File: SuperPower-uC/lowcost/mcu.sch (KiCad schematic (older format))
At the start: 5 parts, among them J5 main pin header, J6 main pin header, U13 ESP32-WROOM32

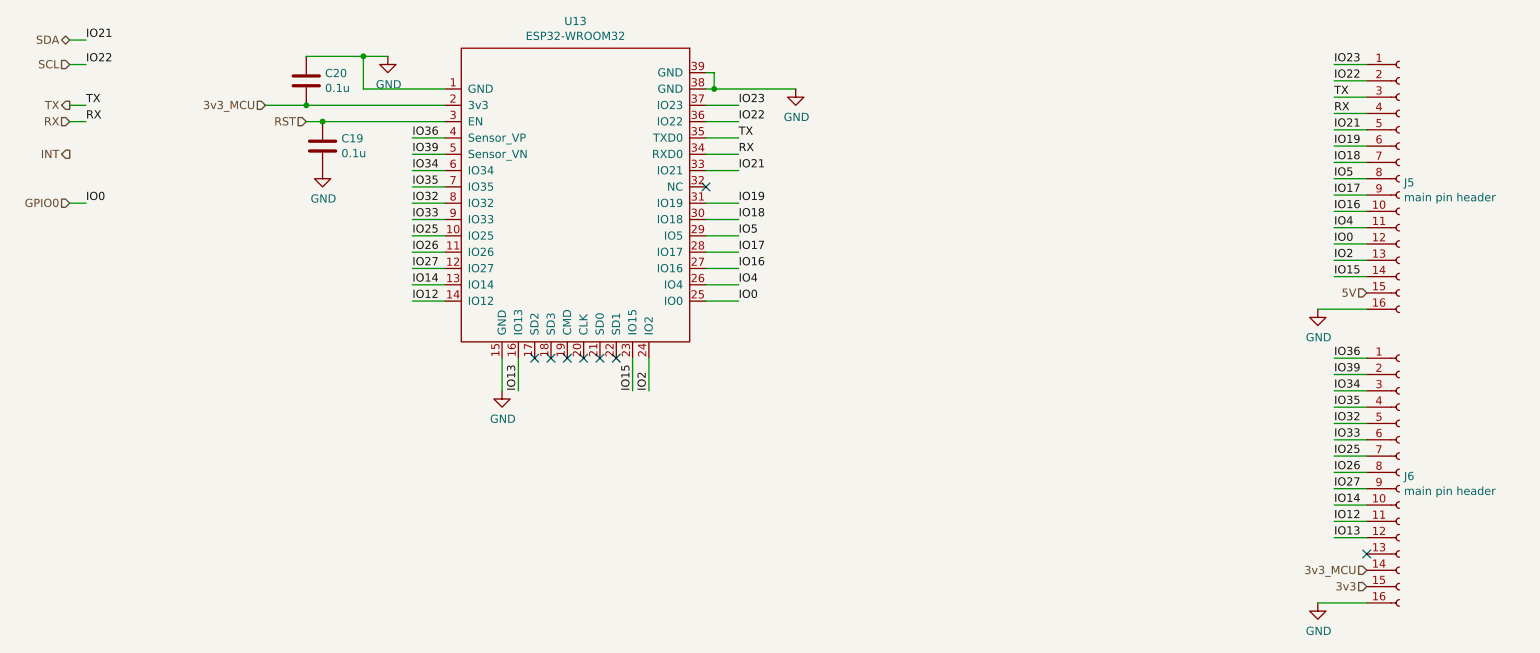
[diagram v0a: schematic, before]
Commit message: design rule optimisation
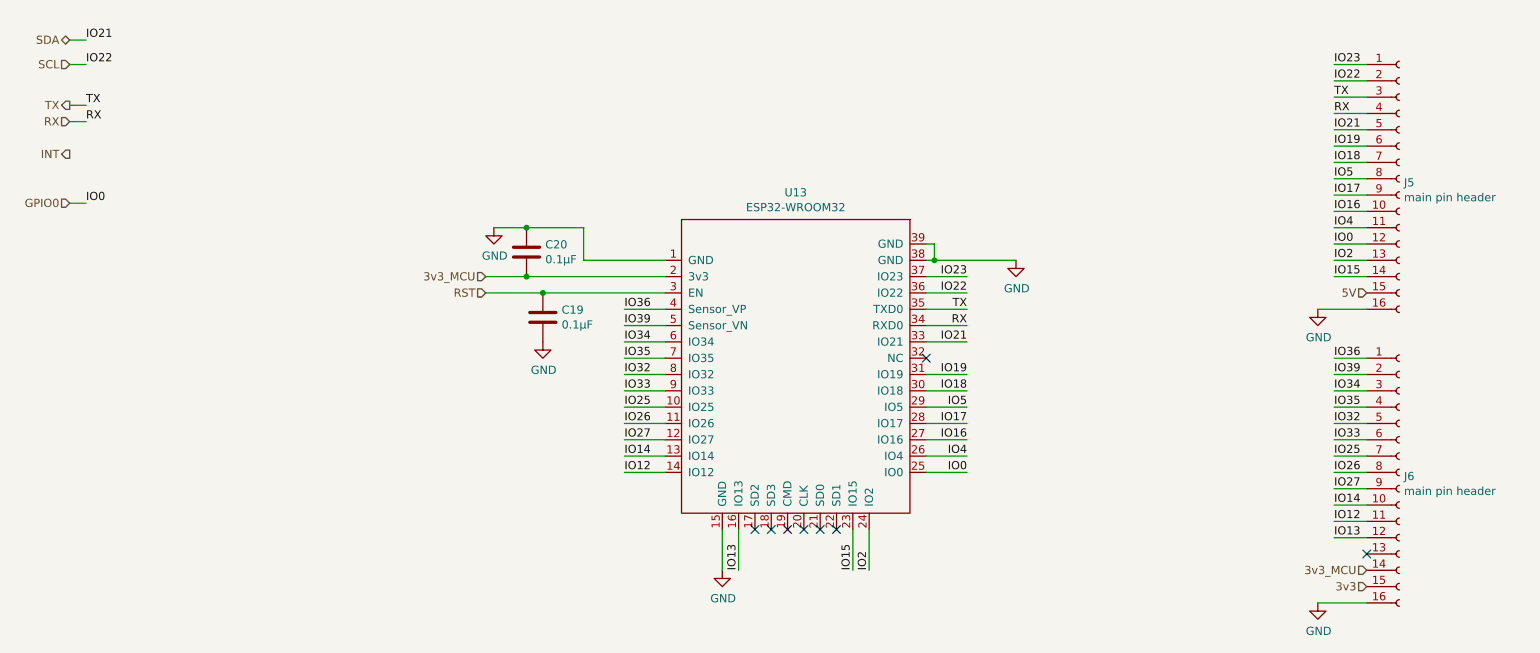
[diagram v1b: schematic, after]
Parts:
- C19, C20: value 0.1u -> 0.1µF
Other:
- moved on the sheet: C19, C20, U13
